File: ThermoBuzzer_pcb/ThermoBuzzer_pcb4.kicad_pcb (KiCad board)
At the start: 2 copper layers, 61 x 59.7 mm, 10 parts, among them SW2 SW_Push

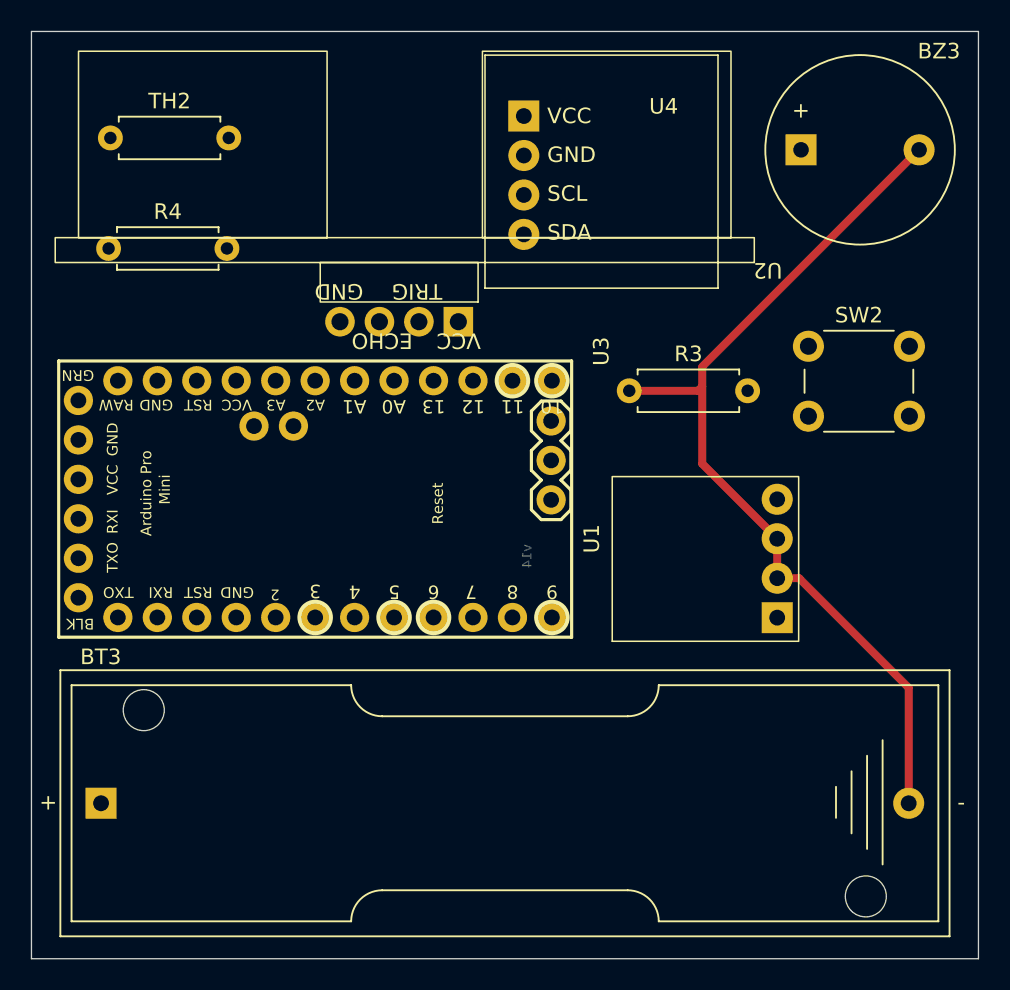
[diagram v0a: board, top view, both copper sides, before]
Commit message: 4.23
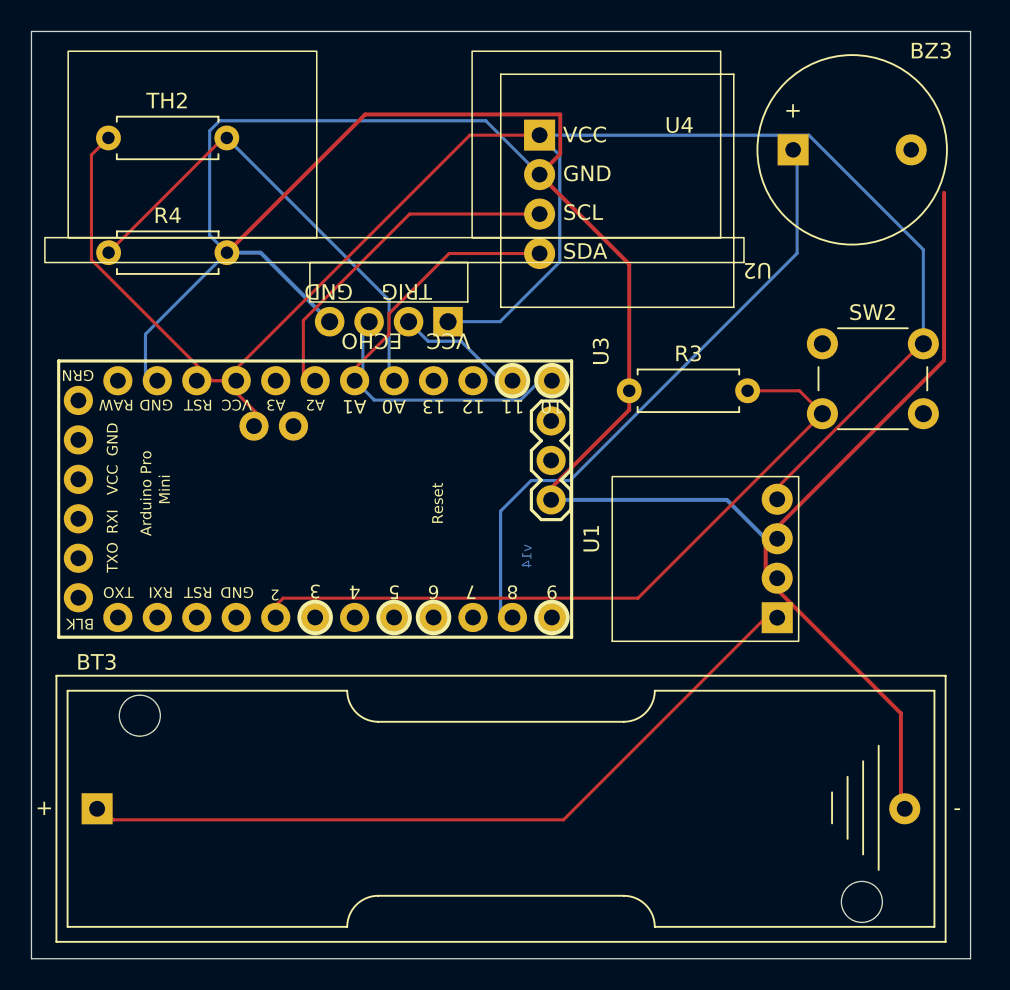
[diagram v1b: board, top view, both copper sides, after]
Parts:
- moved U4 1.59 mm to (131.2, 79.3)
- moved SW2 0.91 mm to (144.9, 88.7)
- moved U2 0.66 mm to (139.8, 83.5)
- moved BZ3 0.51 mm to (143.0, 76.2)
- moved BT3 0.44 mm to (98.2, 118.6)
- moved R4 0.27 mm to (98.9, 82.8)
- moved TH2 0.12 mm to (98.9, 75.4)
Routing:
- net +3.3V: track 0.00 -> 115.9 mm
- net GND: track 59.0 -> 126.8 mm
- net +1.5V: track 0.00 -> 49.2 mm
- net Net-(U1-2): track 0.00 -> 46.8 mm
- net Net-(U4-GND): track 0.00 -> 40.8 mm
- net Net-(BZ3-+): track 0.00 -> 38.6 mm
- net Net-(U1-A0): track 0.00 -> 30.8 mm
- net Net-(U1-A2): track 0.00 -> 21.9 mm
- net Net-(U1-A1): track 0.00 -> 16.8 mm
- net Net-(U1-10): track 0.00 -> 16.7 mm
- net Net-(U1-11): track 0.00 -> 7.50 mm
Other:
- board size 61 x 59.7 mm -> 60.5 x 59.7 mm
